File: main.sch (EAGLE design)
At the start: 36 parts, among them IC1 ATTINY13A-SSH, IC2 TP4056-42-ESOP8, IC3 LM27313XMFX_NOPB, T1A 2N4401, T1B NPN, X1 MINI-USB-UX60A-MB-5ST, X2 332-02

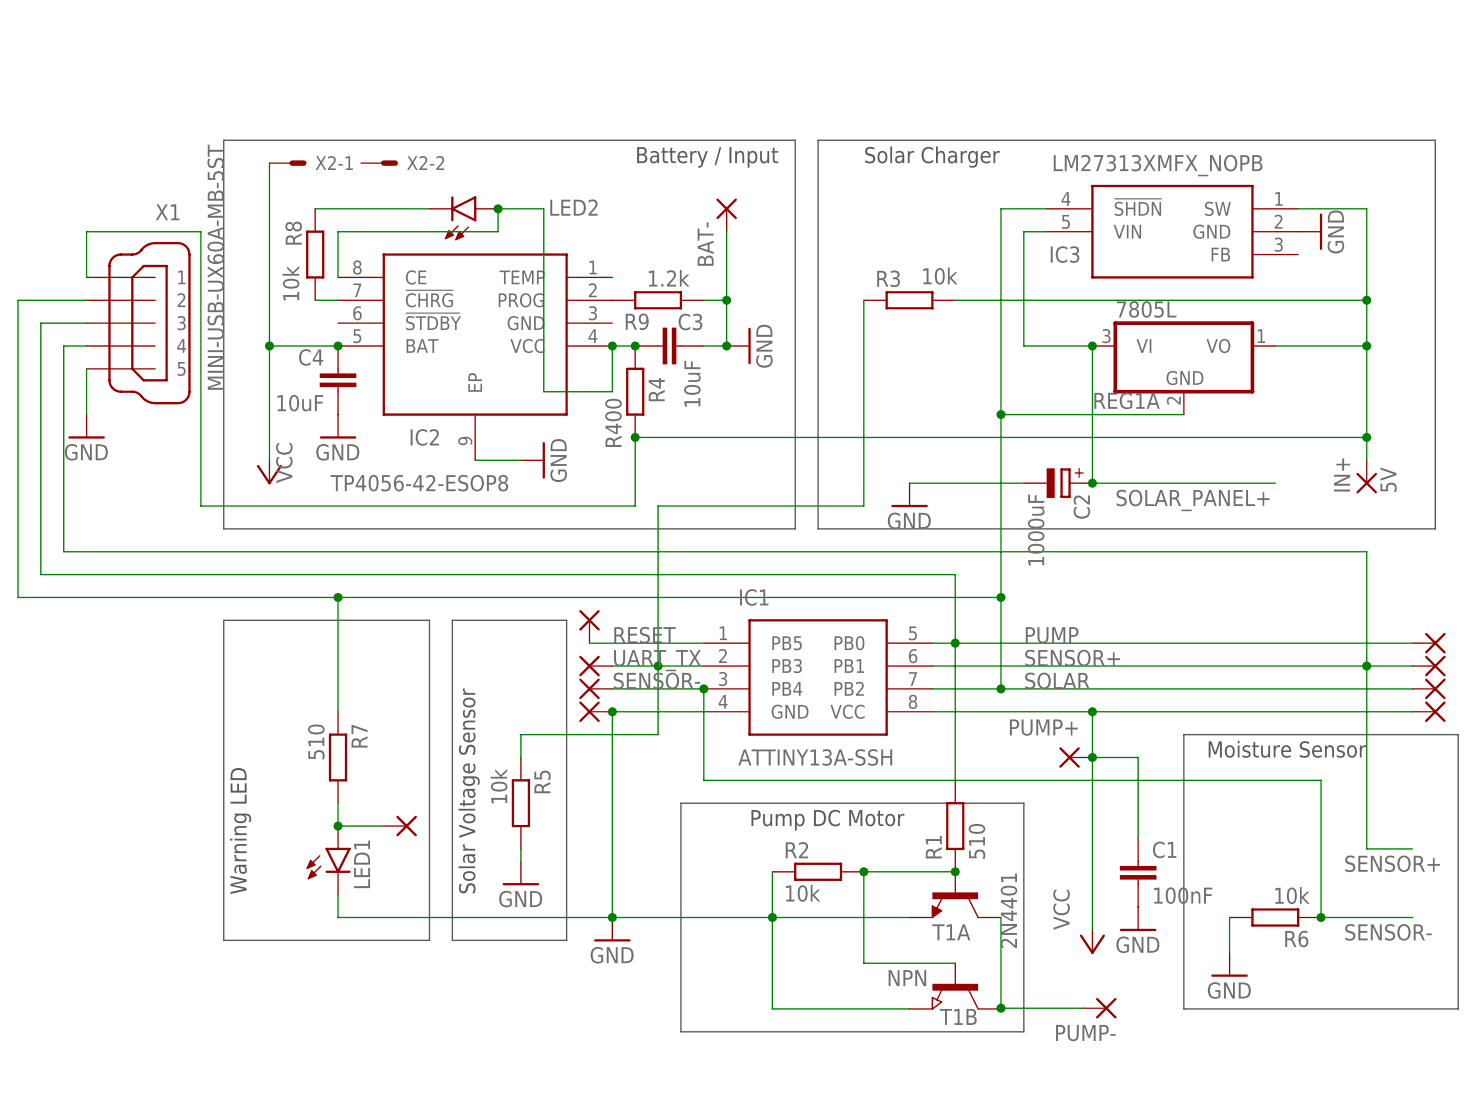
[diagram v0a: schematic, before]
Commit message: improved solar
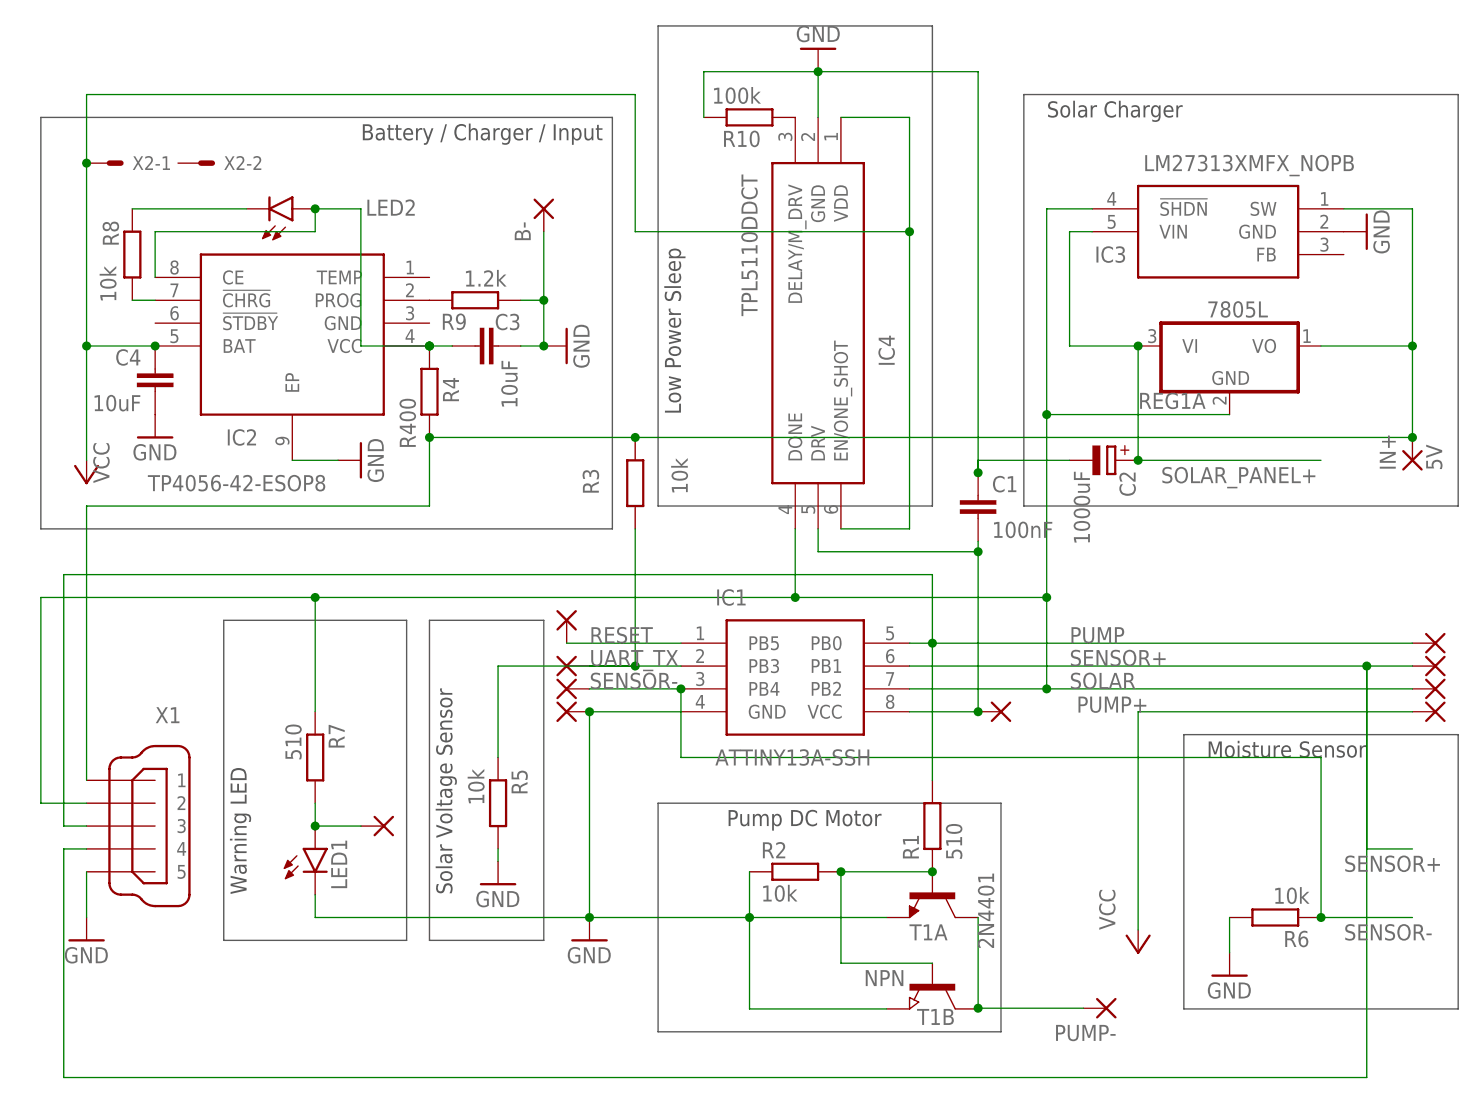
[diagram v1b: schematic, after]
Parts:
- removed BAT-: (no value), wirepad:1,6/0,8
- added B-: (no value), wirepad:1,6/0,8
- added IC4: TPL5110DDCT, SamacSys:TPL5110DDCT
- added R10: 100k, resistor:R-EU_M0805
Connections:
- new net N$3: C1.2, IC1.VCC, IC4.DRV, PAD3.P
- new net N$7: IC4.DELAY/M_DRV, R10.1
- net GND: now also B-.P, C1.1, IC4.GND, R10.2; no longer BAT-.P, C1.2
- net SOLAR: now also IC4.DONE
- net VCC: now also IC4.EN/ONE_SHOT, IC4.VDD; no longer C1.1, IC1.VCC, PAD3.P
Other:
- note added: "Battery / Charger / Input"
- note added: "Low Power Sleep"
- note removed: "Battery / Input"
- moved on the sheet: C1, C2, C3, C4, IC1, IC2, IC3, IN+, LED1, LED2, R1, R2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
